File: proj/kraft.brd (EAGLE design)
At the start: 14 x 20.3 mm, 10 parts, among them J1 TERMBLK_235, J2 TERMBLK_235, P1 PIN_5, P2 PIN_5

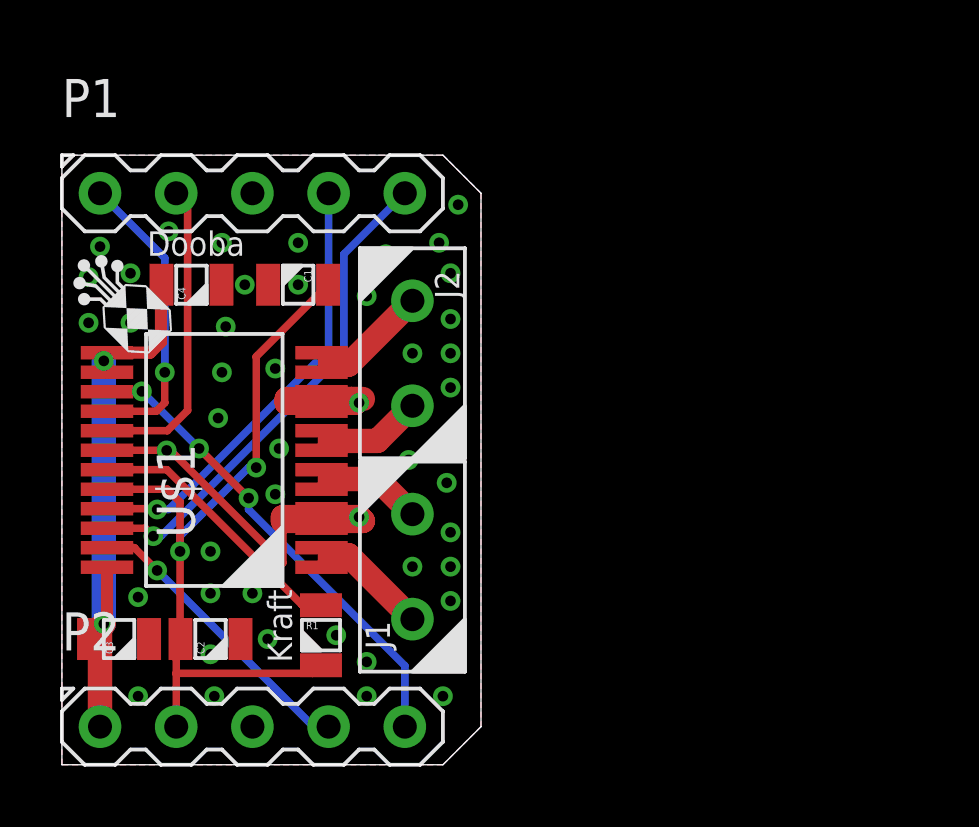
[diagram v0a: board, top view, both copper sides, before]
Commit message: Completed Kraft Board
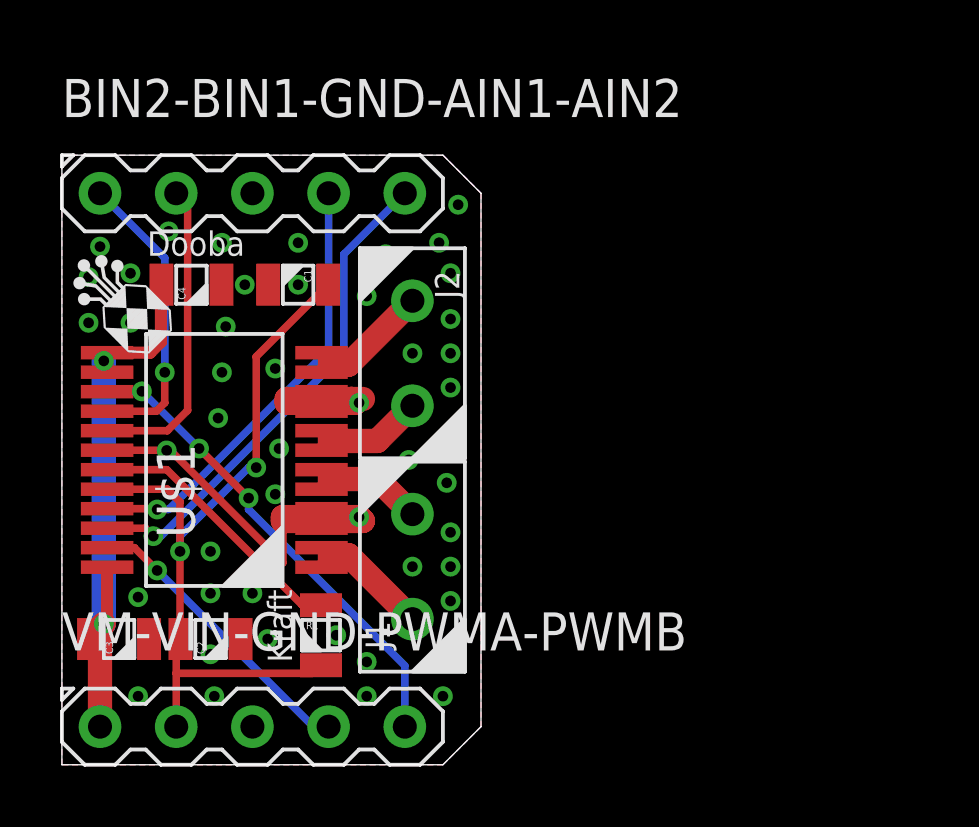
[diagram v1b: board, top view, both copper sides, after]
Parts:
- renumbered P1 to BIN2-BIN1-GND-AIN1-AIN2, P2 to VM-VIN-GND-PWMA-PWMB
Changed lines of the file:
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@@
 <layer number="25" name="tNames" color="7" fill="1" visible="no" active="yes"/>
 <layer number="26" name="bNames" color="7" fill="1" visible="no" active="yes"/>
-<layer number="27" name="tValues" color="7" fill="1" visible="no" active="yes"/>
+<layer number="27" name="tValues" color="7" fill="1" visible="yes" active="yes"/>
 <layer number="28" name="bValues" color="7" fill="1" visible="no" active="yes"/>
 <layer number="29" name="tStop" color="7" fill="3" visible="no" active="yes"/>
@@
 <element name="J1" library="dooba" package="TERMBLK_35_2" value="TERMBLK_235" x="40.894" y="35.814" rot="R90"/>
 <element name="J2" library="dooba" package="TERMBLK_35_2" value="TERMBLK_235" x="40.894" y="42.926" rot="R270"/>
-<element name="P1" library="dooba" package="PIN_5" value="PIN_5" x="35.56" y="48.26"/>
-<element name="P2" library="dooba" package="PIN_5" value="PIN_5" x="35.56" y="30.48"/>
+<element name="BIN2-BIN1-GND-AIN1-AIN2" library="dooba" package="PIN_5" value="PIN_5" x="35.56" y="48.26"/>
+<element name="VM-VIN-GND-PWMA-PWMB" library="dooba" package="PIN_5" value="PIN_5" x="35.56" y="30.48"/>
 <element name="R1" library="dooba" package="0805" value="10k" x="37.846" y="33.528" rot="R270"/>
 <element name="U$1" library="dooba" package="SSOP24" value="TB6612SSOP24" x="34.29" y="39.37" rot="R90"/>
@@
 <contactref element="C3" pad="2"/>
 <contactref element="C4" pad="2"/>
-<contactref element="P1" pad="3"/>
-<contactref element="P2" pad="3"/>
+<contactref element="BIN2-BIN1-GND-AIN1-AIN2" pad="3"/>
+<contactref element="VM-VIN-GND-PWMA-PWMB" pad="3"/>
 <polygon width="0.254" layer="1" isolate="0.3048">
 <vertex x="29.21" y="49.53"/>
@@
 <contactref element="C1" pad="1"/>
 <contactref element="R1" pad="2"/>
-<contactref element="P2" pad="2"/>
+<contactref element="VM-VIN-GND-PWMA-PWMB" pad="2"/>
 <wire x1="33.02" y1="30.48" x2="33.02" y2="32.258" width="0.254" layer="1"/>
 <wire x1="33.02" y1="32.258" x2="33.02" y2="33.258" width="0.254" layer="1"/>
@@
 <contactref element="C3" pad="1"/>
 <contactref element="C4" pad="1"/>
-<contactref element="P2" pad="1"/>
+<contactref element="VM-VIN-GND-PWMA-PWMB" pad="1"/>
 <wire x1="30.715" y1="42.945" x2="32.15" y2="42.945" width="0.4064" layer="1"/>
 <wire x1="32.15" y1="42.945" x2="32.512" y2="43.307" width="0.4064" layer="1"/>
@@
 <signal name="N$4">
 <contactref element="U$1" pad="15"/>
-<contactref element="P2" pad="5"/>
+<contactref element="VM-VIN-GND-PWMA-PWMB" pad="5"/>
 <wire x1="30.715" y1="41.645" x2="31.866" y2="41.645" width="0.254" layer="1"/>
 <wire x1="31.866" y1="41.645" x2="31.877" y2="41.656" width="0.254" layer="1"/>
@@
 <signal name="N$6">
 <contactref element="U$1" pad="22"/>
-<contactref element="P1" pad="5"/>
+<contactref element="BIN2-BIN1-GND-AIN1-AIN2" pad="5"/>
 <wire x1="30.715" y1="37.095" x2="31.993" y2="37.095" width="0.254" layer="1"/>
 <wire x1="31.993" y1="37.095" x2="32.258" y2="36.83" width="0.254" layer="1"/>
@@
 </signal>
 <signal name="N$5">
-<contactref element="P1" pad="4"/>
+<contactref element="BIN2-BIN1-GND-AIN1-AIN2" pad="4"/>
 <contactref element="U$1" pad="21"/>
 <wire x1="30.715" y1="37.745" x2="32.359" y2="37.745" width="0.254" layer="1"/>
@@
 </signal>
 <signal name="N$7">
-<contactref element="P1" pad="2"/>
+<contactref element="BIN2-BIN1-GND-AIN1-AIN2" pad="2"/>
 <contactref element="U$1" pad="17"/>
 <wire x1="30.715" y1="40.345" x2="32.725" y2="40.345" width="0.254" layer="1"/>
@@
 </signal>
 <signal name="N$8">
-<contactref element="P1" pad="1"/>
+<contactref element="BIN2-BIN1-GND-AIN1-AIN2" pad="1"/>
 <contactref element="U$1" pad="16"/>
 <wire x1="30.48" y1="48.26" x2="32.639" y2="46.101" width="0.254" layer="16"/>
@@
 </signal>
 <signal name="N$3">
-<contactref element="P2" pad="4"/>
+<contactref element="VM-VIN-GND-PWMA-PWMB" pad="4"/>
 <contactref element="U$1" pad="23"/>
 <wire x1="30.715" y1="36.445" x2="31.627" y2="36.445" width="0.254" layer="1"/>
